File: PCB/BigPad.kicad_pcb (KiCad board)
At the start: 2 copper layers, 190.5 x 59.7 mm, 33 parts, among them SW1 RotaryEncoder_Switch, SW2 RotaryEncoder_Switch

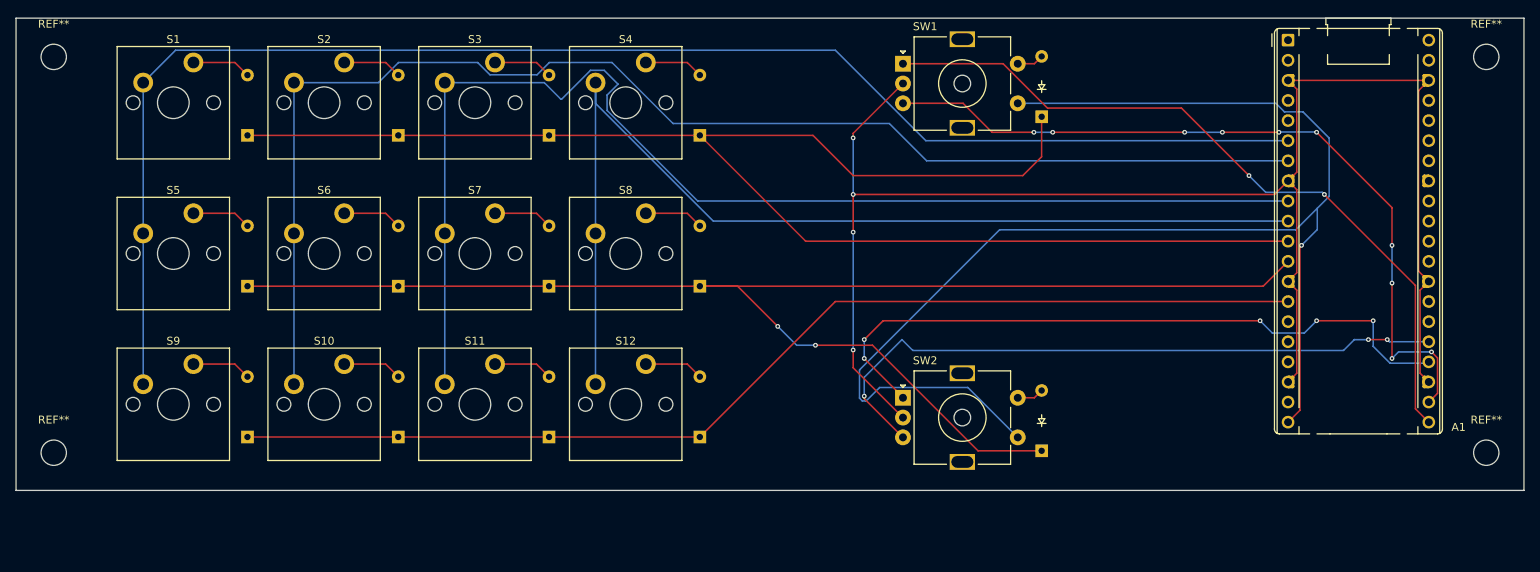
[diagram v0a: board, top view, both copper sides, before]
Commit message: fixed several wiring issues
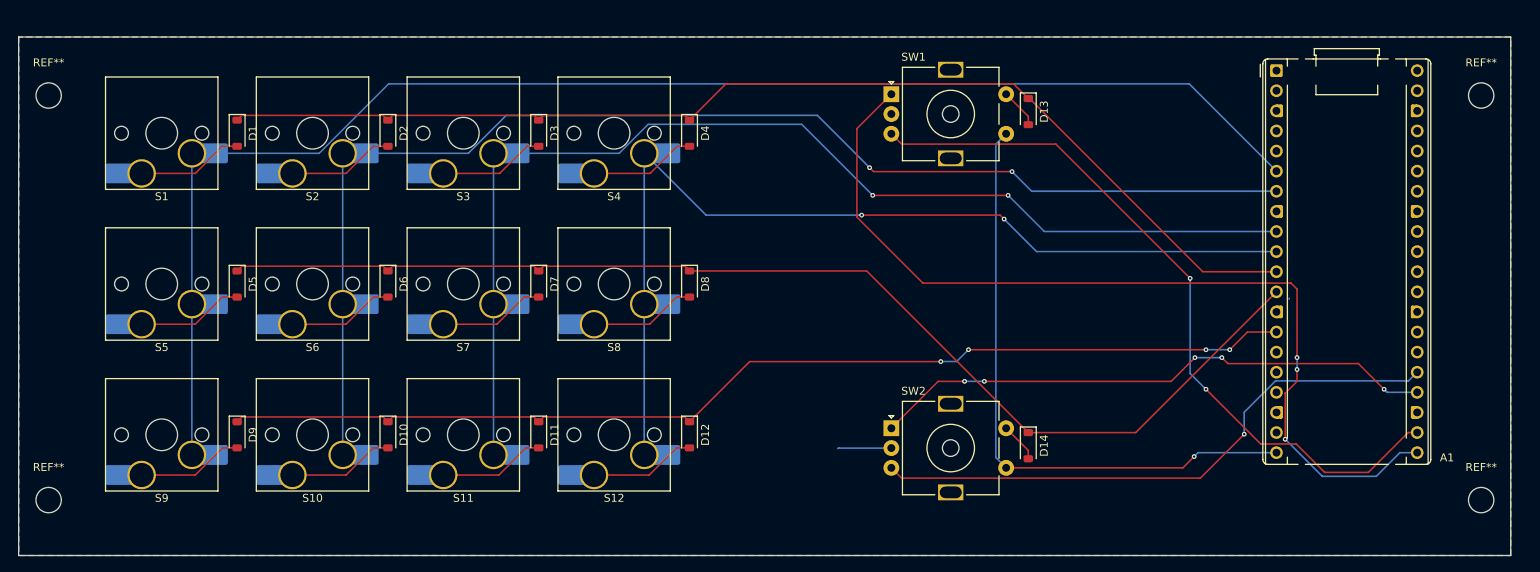
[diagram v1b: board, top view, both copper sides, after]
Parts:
- removed the REF** at (47.6, 76.2)
- removed the REF** at (47.6, 126.2)
- removed the REF** at (228.6, 76.2)
- removed the REF** at (228.6, 126.2)
- added REF**: MountingHole_3.2mm_M3, MountingHole:MountingHole_3.2mm_M3, F.Cu at (47.0, 81.1)
- added REF**: MountingHole_3.2mm_M3, MountingHole:MountingHole_3.2mm_M3, F.Cu at (47.0, 132.2)
- added REF**: MountingHole_3.2mm_M3, MountingHole:MountingHole_3.2mm_M3, F.Cu at (228.0, 81.1)
- added REF**: MountingHole_3.2mm_M3, MountingHole:MountingHole_3.2mm_M3, F.Cu at (228.0, 132.2)
- D1, D10, D11, D12, D2, D3, D4, D5, D6, D7, D8, D9: footprint ScottoKeebs_Components:Diode_DO-35 -> Diode_SMD:D_SOD-123; moved to F.Cu
- D13, D14: footprint ScottoKeebs_Components:Diode_DO-35 -> Diode_SMD:D_SOD-123
- S1, S10, S11, S12, S2, S3, S4, S5, S6, S7, S8, S9: footprint ScottoKeebs_MX:MX_PCB_1.00u -> PCM_Switch_Keyboard_Hotswap_Kailh:SW_Hotswap_Kailh_MX_Plated_1.00u
- moved S1 4.12 mm to (61.3, 85.8), turned to 180 degrees
- moved S2 4.12 mm to (80.3, 85.8), turned to 180 degrees
- moved S4 4.12 mm to (118.4, 85.8), turned to 180 degrees
- moved SW1 4.12 mm to (153.4, 80.9)
- moved SW2 4.12 mm to (153.4, 123.1)
- moved S3 4.12 mm to (99.4, 85.8), turned to 180 degrees
- moved S10 4.12 mm to (80.3, 123.9), turned to 180 degrees
- moved S12 4.12 mm to (118.4, 123.9), turned to 180 degrees
- moved S5 4.12 mm to (61.3, 104.9), turned to 180 degrees
- moved S6 4.12 mm to (80.3, 104.9), turned to 180 degrees
- moved S8 4.12 mm to (118.4, 104.9), turned to 180 degrees
- moved S9 4.12 mm to (61.3, 123.9), turned to 180 degrees
- moved S11 4.12 mm to (99.4, 123.9), turned to 180 degrees
- moved S7 4.12 mm to (99.4, 104.9), turned to 180 degrees
- moved A1 4.12 mm to (202.1, 77.9)
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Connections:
- net Net-(A1-GND-Pad13) renamed GND
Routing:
- net GND: track 201.8 -> 7.03 mm, vias 4 -> 0
- net /Column 4: track 172.5 -> 78.2 mm
- net /Row 0: track 188.3 -> 144.5 mm
- net /Row 1: track 184.6 -> 148.6 mm, vias 2 -> 0
- net Net-(A1-GPIO16): track 94.3 -> 116.5 mm, vias 2 -> 3
- net Net-(A1-GPIO18): track 87.2 -> 71.9 mm
- net /Column 2: track 157.7 -> 144.1 mm, vias 0 -> 2
- net /Column 3: track 134.4 -> 123.1 mm, vias 0 -> 2
- net Net-(A1-GPIO19): track 84.2 -> 74.1 mm, vias 3 -> 1
- net /Column 1: track 171.2 -> 162.0 mm, vias 0 -> 2
- net Net-(D9-A): track 7.48 -> 13.5 mm
- net Net-(D5-A): track 7.48 -> 13.5 mm
- net Net-(D10-A): track 7.48 -> 13.5 mm
- net Net-(D1-A): track 7.48 -> 13.5 mm
- net Net-(D12-A): track 7.48 -> 13.5 mm
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- added copper zone on B.Cu, net GND
- added copper zone on F.Cu, net GND
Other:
- board size 190.5 x 59.7 mm -> 188.5 x 65.5 mm
